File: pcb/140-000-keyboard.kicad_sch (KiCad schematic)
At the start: 13 parts, among them SW42 SW_Push, U3 ATmega32U4-A, U5 RP2040, Y1 16MHz

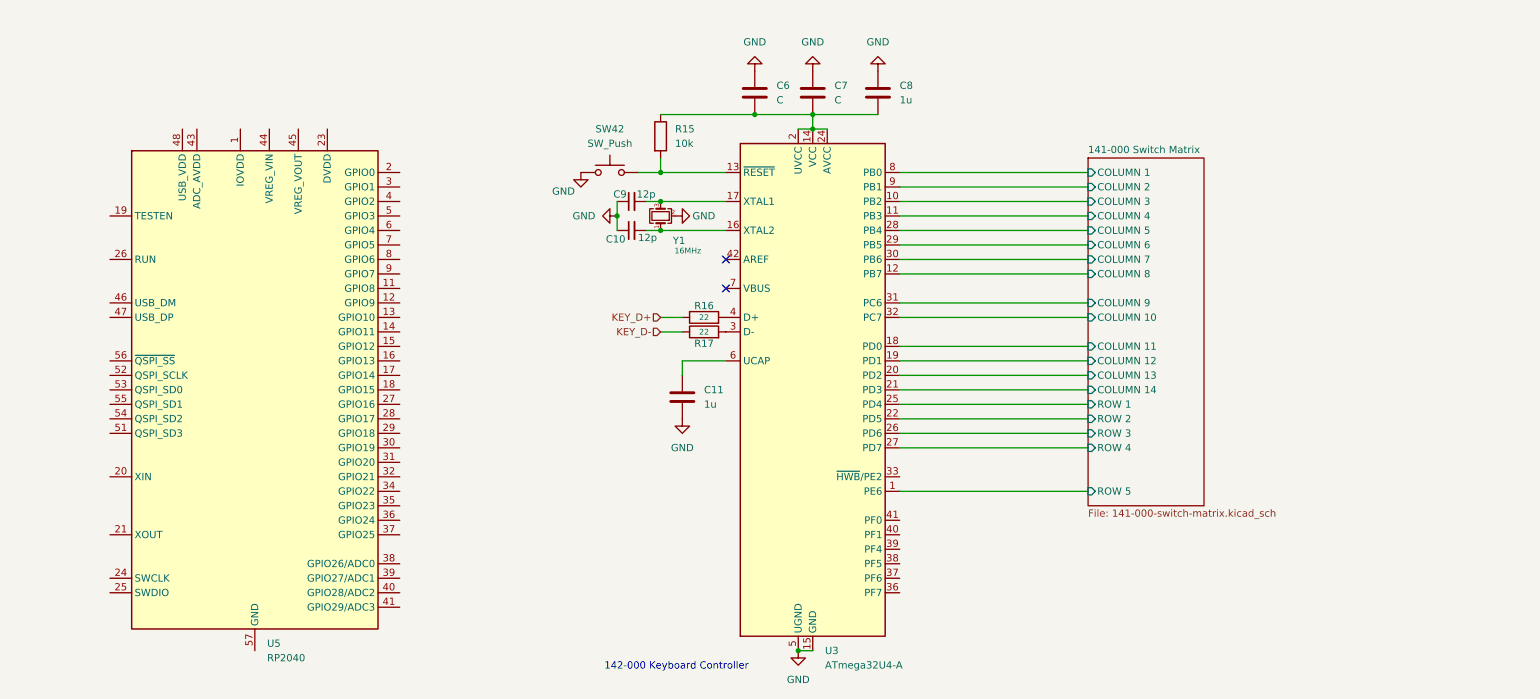
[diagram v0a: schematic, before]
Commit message: add git ignore, and new sheets etc
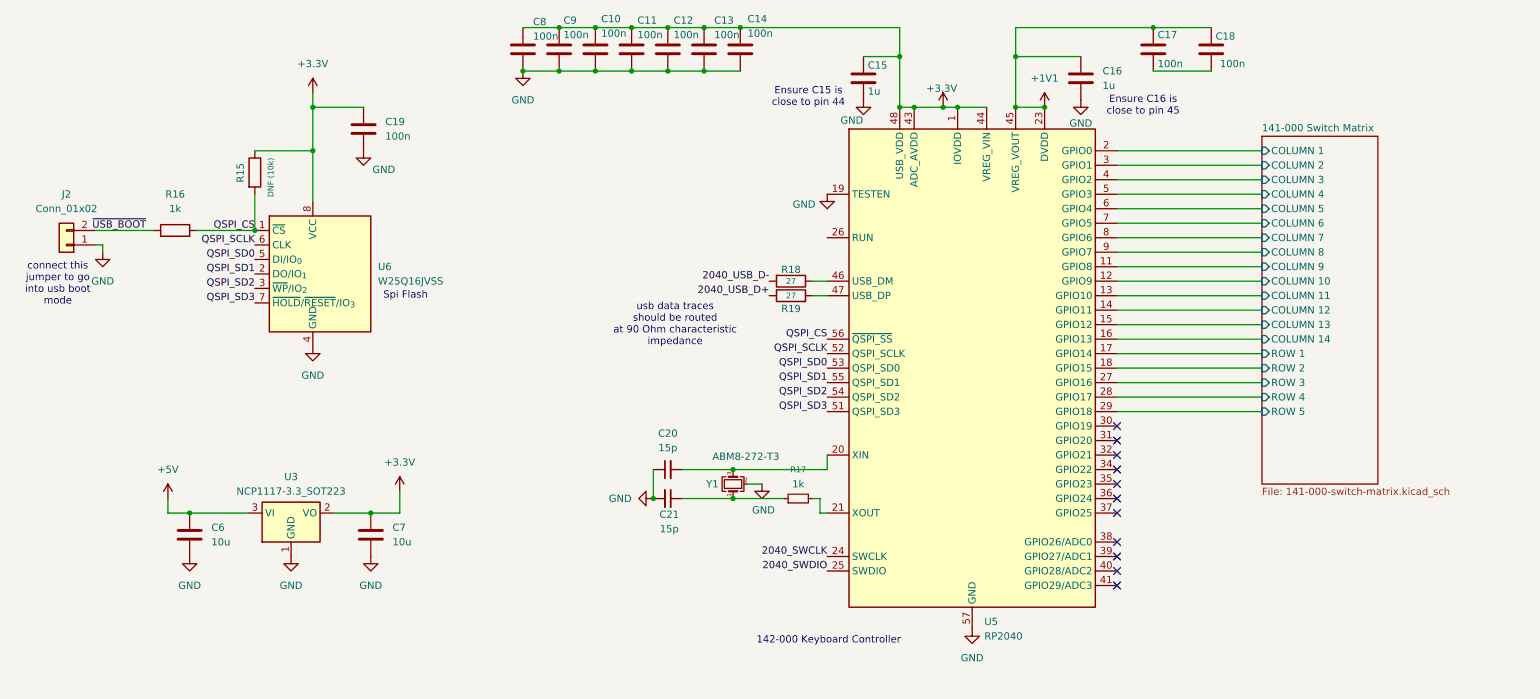
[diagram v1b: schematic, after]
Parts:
- removed C10, C9: 12p, symbol Device:C_Small
- removed R17: 22, symbol Device:R
- removed SW42: SW_Push, Kahil Switches:SW_Kailh_Choc_Mini_2.25u, symbol Switch:SW_Push
- removed U3: ATmega32U4-A, Package_QFP:TQFP-44_10x10mm_P0.8mm, symbol MCU_Microchip_ATmega:ATmega32U4-A
- added C10, C12, C13, C14, C17, C18, C19, C9: 100n, symbol Device:C
- added C15, C16: 1u, symbol Device:C
- added C20, C21: 15p, symbol Device:C_Small
- added J2: Conn_01x02, symbol Connector_Generic:Conn_01x02
- added R17: 1k, symbol Device:R_Small
- added R18, R19: 27, symbol Device:R
- added U3: NCP1117-3.3_SOT223, Package_TO_SOT_SMD:SOT-223-3_TabPin2, symbol Regulator_Linear:NCP1117-3.3_SOT223
- added U6: W25Q16JVSS, Package_SO:SOIC-8_5.3x5.3mm_P1.27mm, symbol Memory_Flash:W25Q16JVSS
- C11, C8: value 1u -> 100n
- C6, C7: value C -> 10u
- R15: value 10k -> DNF (10k)
- R16: value 22 -> 1k
- Y1: value 16MHz -> ABM8-272-T3; footprint (none) -> perpetusest-parts:ABM8-272-T3_ABR
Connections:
- net 141-000 Switch Matrix/COLUMN 1: now also U5.2 (GPIO0)
- net 141-000 Switch Matrix/COLUMN 10: now also U5.12 (GPIO9)
- net 141-000 Switch Matrix/COLUMN 11: now also U5.13 (GPIO10)
- net 141-000 Switch Matrix/COLUMN 12: now also U5.14 (GPIO11)
- net 141-000 Switch Matrix/COLUMN 13: now also U5.15 (GPIO12)
- net 141-000 Switch Matrix/COLUMN 14: now also U5.16 (GPIO13)
- net 141-000 Switch Matrix/COLUMN 2: now also U5.3 (GPIO1)
- net 141-000 Switch Matrix/COLUMN 3: now also U5.4 (GPIO2)
- net 141-000 Switch Matrix/COLUMN 4: now also U5.5 (GPIO3)
- net 141-000 Switch Matrix/COLUMN 5: now also U5.6 (GPIO4)
- net 141-000 Switch Matrix/COLUMN 6: now also U5.7 (GPIO5)
- net 141-000 Switch Matrix/COLUMN 7: now also U5.8 (GPIO6)
- net 141-000 Switch Matrix/COLUMN 8: now also U5.9 (GPIO7)
- net 141-000 Switch Matrix/COLUMN 9: now also U5.11 (GPIO8)
- net 141-000 Switch Matrix/ROW 1: now also U5.17 (GPIO14)
- net 141-000 Switch Matrix/ROW 2: now also U5.18 (GPIO15)
- net 141-000 Switch Matrix/ROW 3: now also U5.27 (GPIO16)
- net 141-000 Switch Matrix/ROW 4: now also U5.28 (GPIO17)
- net 141-000 Switch Matrix/ROW 5: now also U5.29 (GPIO18)
- net GND: now also C6.2, C7.2, C8.2, U5.19 (TESTEN), U5.57 (GND), C10.2, C12.2, C13.2, C14.2, C15.2, C16.2, C19.2, C20.1, C21.2, C9.2, J2.1 (Pin_1), U3.1 (GND), U6.4 (GND); no longer C6.1, C7.1, C8.1
- net QSPI_CS: now reaches R15.2
- net QSPI_CS: now also R16.2, U5.56 (~{QSPI_SS}), U6.1 (~{CS})
- net at Y1.1: now also C21.1, R17.1
- net at Y1.3: now also U5.20 (XIN), C20.2
- net +3.3V: now reaches U5.1 (IOVDD), U5.10 (IOVDD), U5.22 (IOVDD), U5.33 (IOVDD), U5.42 (IOVDD), U5.49 (IOVDD)
- net +3.3V: now also C11.1, C7.1, C8.1, R15.1, U5.43 (ADC_AVDD), U5.44 (VREG_VIN), U5.48 (USB_VDD), C10.1, C12.1, C13.1, C14.1, C15.1, C19.1, C9.1, U3.2 (VO), U6.8 (VCC)
- net at U5.21 (XOUT): now also R17.2
- net +1V1: now reaches U5.23 (DVDD), U5.50 (DVDD)
- net +1V1: now also U5.45 (VREG_VOUT), C16.1, C17.1, C18.1
- net 2040_SWCLK: now reaches U5.24 (SWCLK)
- net 2040_SWDIO: now reaches U5.25 (SWDIO)
- net at U5.46 (USB_DM): now also R18.1
- net at U5.47 (USB_DP): now also R19.2
- net QSPI_SD3: now reaches U5.51 (QSPI_SD3)
- net QSPI_SD3: now also U6.7 (~{HOLD}/~{RESET}/IO_{3})
- net QSPI_SCLK: now reaches U5.52 (QSPI_SCLK)
- net QSPI_SCLK: now also U6.6 (CLK)
- net QSPI_SD0: now reaches U5.53 (QSPI_SD0)
- net QSPI_SD0: now also U6.5 (DI/IO_{0})
- net QSPI_SD2: now reaches U5.54 (QSPI_SD2)
- net QSPI_SD2: now also U6.3 (~{WP}/IO_{2})
- net QSPI_SD1: now reaches U5.55 (QSPI_SD1)
- net QSPI_SD1: now also U6.2 (DO/IO_{1})
- net KEY_D+ renamed ~{USB_BOOT}
- net ~{USB_BOOT}: now also J2.2 (Pin_2)
- new net: C17.2, C18.2
- new net +5V: C6.1, U3.3 (VI)
- new net 2040_USB_D+: R19.1
- new net 2040_USB_D-: R18.2
- no-connect marks 2 -> 11
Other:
- note added: "Ensure C15 is close to pin 44"
- note added: "Ensure C16 is close to pin 45"
- note added: "Spi Flash"
- note added: "connect this jumper to go into usb boot mode"
- note added: "usb data traces should be routed at 90 Ohm characteristic impedance"
- moved on the sheet: U5
